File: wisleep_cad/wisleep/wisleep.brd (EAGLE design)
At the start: 53.2 x 54.4 mm, 25 parts, among them IC1 STM32F10XCXT6, X1 8MHz

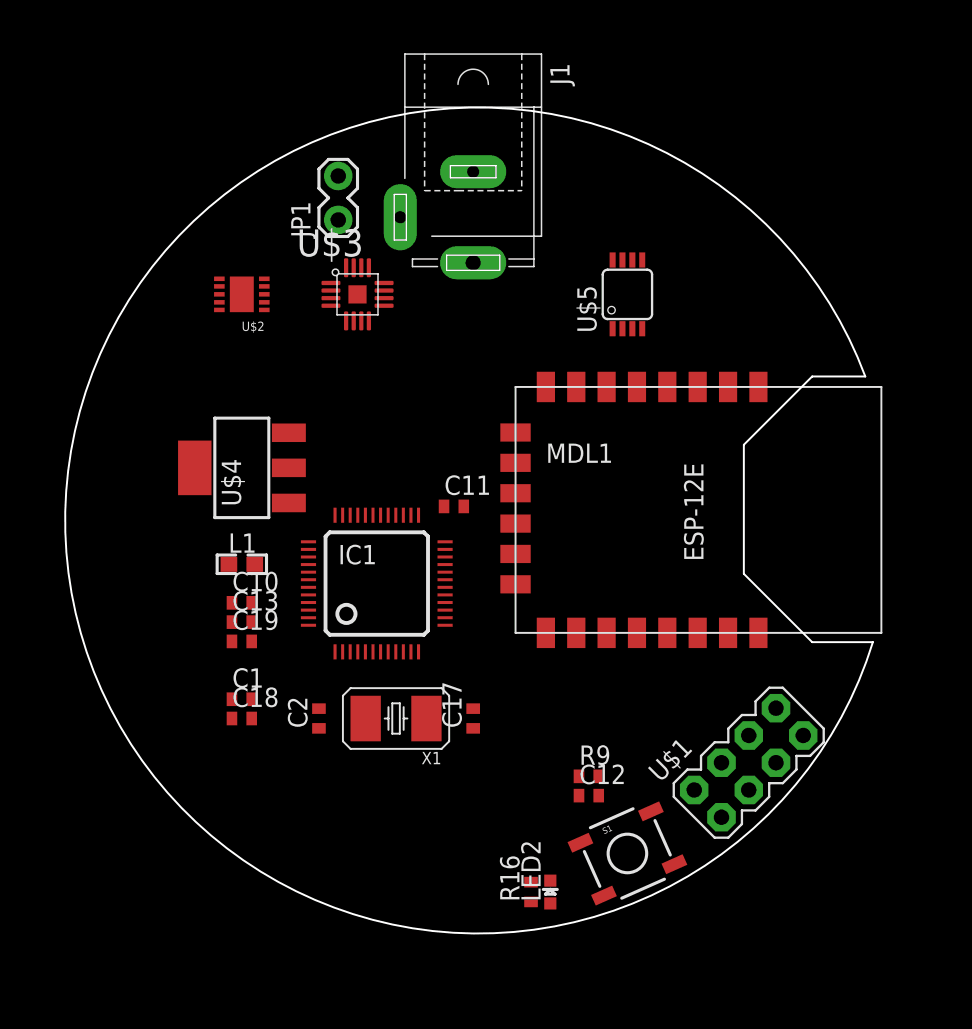
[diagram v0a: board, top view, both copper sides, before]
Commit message: even moar cad
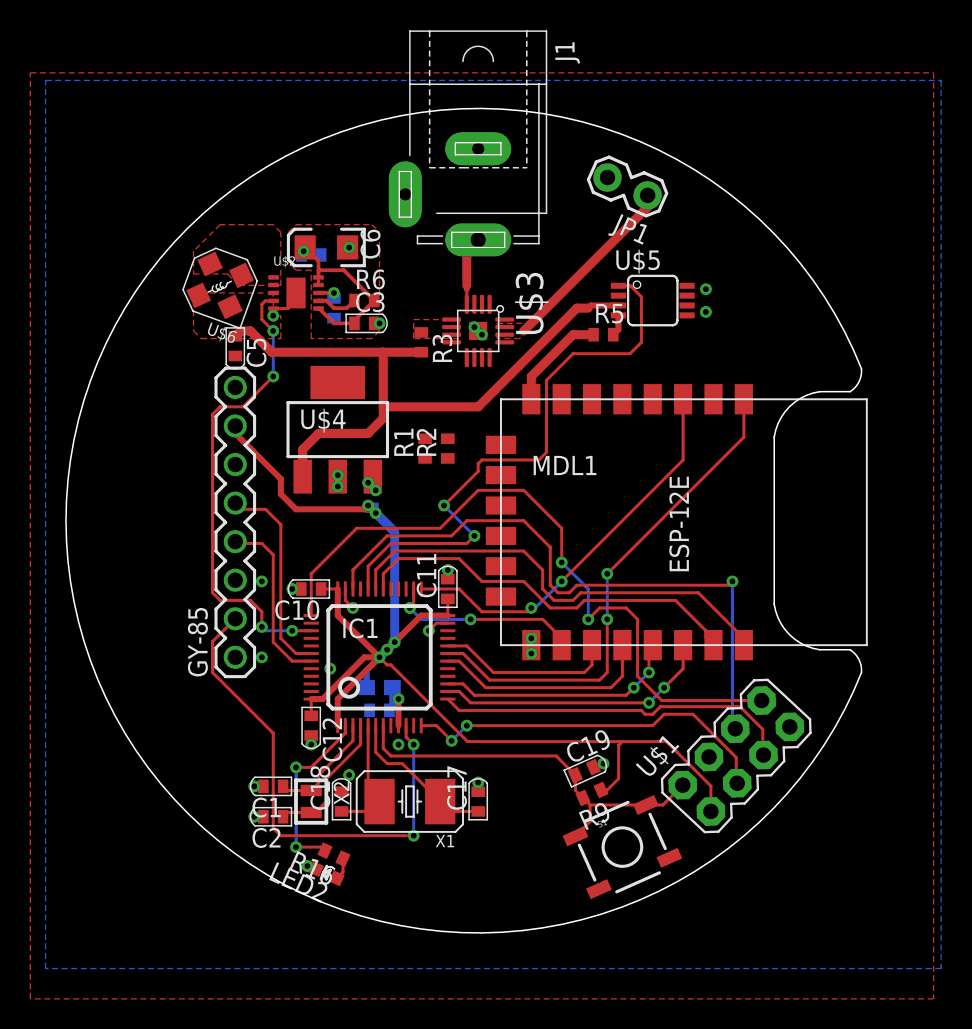
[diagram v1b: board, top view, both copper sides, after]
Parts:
- added C3: 0.1uF, robot:C0402
- added C5: 10uF, robot:C0402
- added C6: 22uF, robot:EIA3216
- added GY-85: (no value), robot:1X08
- added R1, R2, R6, R7: 100k, SparkFunEagle-6-6-07:C0402
- added R3, R4, R5, R8: 0, SparkFunEagle-6-6-07:C0402
- added U$6: (no value), robot:INDUCTOR-3014
- added X2: 32kHz, robot:CRYSTAL_SMD_2X0.6
- U$2: value MAX8815AOWNMAX8815A -> MAX8815A10TDFNEP
- moved C19 24.1 mm to (34.0, 10.5), turned to 24 degrees
- moved JP1 20.3 mm to (38.0, 48.5), turned to 156 degrees
- moved C12 18.9 mm to (16.0, 13.5), turned to 270 degrees
- moved LED2 14.8 mm to (17.0, 3.75), turned to 66 degrees
- moved R16 13.2 mm to (17.5, 5.00), turned to 156 degrees
- moved L1 12.2 mm to (20.5, 16.0), flipped to the bottom, turned to 180 degrees
- moved C13 10.8 mm to (20.5, 14.5), flipped to the bottom
- moved C18 8.55 mm to (18.0, 8.50), turned to 90 degrees
- moved U$3 8.31 mm to (27.0, 39.5), turned to 270 degrees
- moved C2 7.14 mm to (13.5, 7.50), turned to 180 degrees
- moved U$4 6.80 mm to (17.8, 33.0), turned to 0 degrees
- moved C1 6.10 mm to (13.5, 9.50), turned to 180 degrees
- moved X1 5.55 mm to (22.5, 8.50)
- moved C17 5.48 mm to (27.0, 8.50)
- moved C11 5.45 mm to (25.0, 22.5), turned to 90 degrees
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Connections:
- net SPI_MISO renamed N$18
- net SPI_MOSI renamed N$20
- removed net BAT1: U$3.2
- removed net BAT2: U$3.3
- removed net BATT: U$2.3
- removed net IN: U$3.13, U$4.1, U$5.3
- removed net OUT: U$4.3, U$5.4
- removed net OUT1: U$3.10
- removed net OUT2: U$3.11
- removed net PAD_GND: U$3.PAD
- removed net SPI_CS: IC1.14
- removed net SPI_SCK: IC1.15
- removed net SWDCLK: U$1.8
- new net 5V: R8.1
- new net BAT+: JP1.1, U$3.2, U$3.3
- new net BAT-: JP1.2
- new net G_INT(NC): GY-85.1
- new net M_DRDY(NC): GY-85.3
- new net N$10: U$3.15
- new net N$11: U$3.12
- new net N$12: U$3.16
- new net N$13: R4.2, U$4.3
- new net N$14: R5.2, U$5.4
- new net N$15: U$2.1, U$2.2, U$6.P$2
- new net N$16: R6.1, U$2.7
- new net N$17: IC1.11
- new net N$19: R7.2, U$2.8
- new net N$21: IC1.27
- new net N$22: IC1.33
- new net N$23: IC1.38
- new net N$26: IC1.41
- new net N$27: IC1.40
- new net N$28: IC1.29
- new net N$4: R3.1, U$3.10, U$3.11
- new net N$6: U$3.4
- new net N$8: U$3.6
- new net N$9: U$3.5
- new net NCHG: IC1.21, R1.2, U$3.9
- new net NPGOOD: IC1.22, R2.2, U$3.7
- new net V+: C5.1, R3.2, U$2.3, U$4.1, U$5.3, U$6.P$1
- new net VCC: MDL1.8, R5.1
- new net WIFI_BL15: IC1.26, MDL1.10
- new net WIFI_BL2: IC1.20, MDL1.11
- new net WIFI_BOOT: IC1.18, MDL1.12
- new net WIFI_ENA: IC1.25, MDL1.3
- new net WIFI_IO4: IC1.15, MDL1.13
- new net WIFI_IO5: IC1.14, MDL1.14
- new net WIFI_POW_ENA: IC1.32, U$5.1
- new net WIFI_RES: IC1.19, MDL1.1
- net 3.3V: now also GY-85.7, R1.1, R2.1, R4.1; no longer LED2.A
- net 5V_ENA: now also IC1.39, U$2.4; no longer IC1.29
- net ACC_INT1: now also GY-85.2
- net GND: now also C3.2, C5.2, C6.C, GY-85.6, LED2.C, MDL1.9, R7.1, U$3.PAD
- net N$1: now also X2.P$1
- net N$2: now also X2.P$2
- net N$3: now also C3.1, C6.A, R6.2, R8.2
- net N$5: now also LED2.A; no longer LED2.C
- net POWDC: now also U$3.13
- net SCL: now also GY-85.5, IC1.42; no longer IC1.21
- net SDA: now also GY-85.4, IC1.43; no longer IC1.22
- net SWCLK: now also U$1.8
- net WIFI_RX: now also MDL1.16
- net WIFI_TX: now also MDL1.15
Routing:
- net 3.3V: track 0.00 -> 81.7 mm, vias 0 -> 5
- net SWCLK: track 0.00 -> 45.7 mm, vias 0 -> 2
- net V+: track 0.00 -> 43.5 mm
- net SWDIO: track 0.00 -> 41.1 mm, vias 0 -> 1
- net WIFI_POW_ENA: track 0.00 -> 37.5 mm, vias 0 -> 2
- net WIFI_RES: track 0.00 -> 33.2 mm, vias 0 -> 2
- net ACC_INT1: track 0.00 -> 33.0 mm, vias 0 -> 2
- net 5V_ENA: track 0.00 -> 30.8 mm, vias 0 -> 4
- net WIFI_RX: track 0.00 -> 30.0 mm
- net RST: track 0.00 -> 26.4 mm
- net WIFI_TX: track 0.00 -> 26.2 mm
- net WIFI_ENA: track 0.00 -> 26.0 mm, vias 0 -> 2
- net USART_TX: track 0.00 -> 24.8 mm, vias 0 -> 2
- net USART_RX: track 0.00 -> 23.7 mm
- net WIFI_IO5: track 0.00 -> 18.3 mm, vias 0 -> 2
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- added copper zone on layer 1, net BAT+
- added copper zone on layer 1, net GND
- added copper zone on layer 16, net GND
- added copper zone on layer 1, net N$15
- added copper zone on layer 1, net N$3
- added copper zone on layer 1, net N$4
- added copper zone on layer 1, net V+
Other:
- board size 53.2 x 54.4 mm -> 52.4 x 54.3 mm
